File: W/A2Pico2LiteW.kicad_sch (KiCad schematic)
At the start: 15 parts, among them J1 SolderJumper_2_Bridged, U1 RPI-Pico2

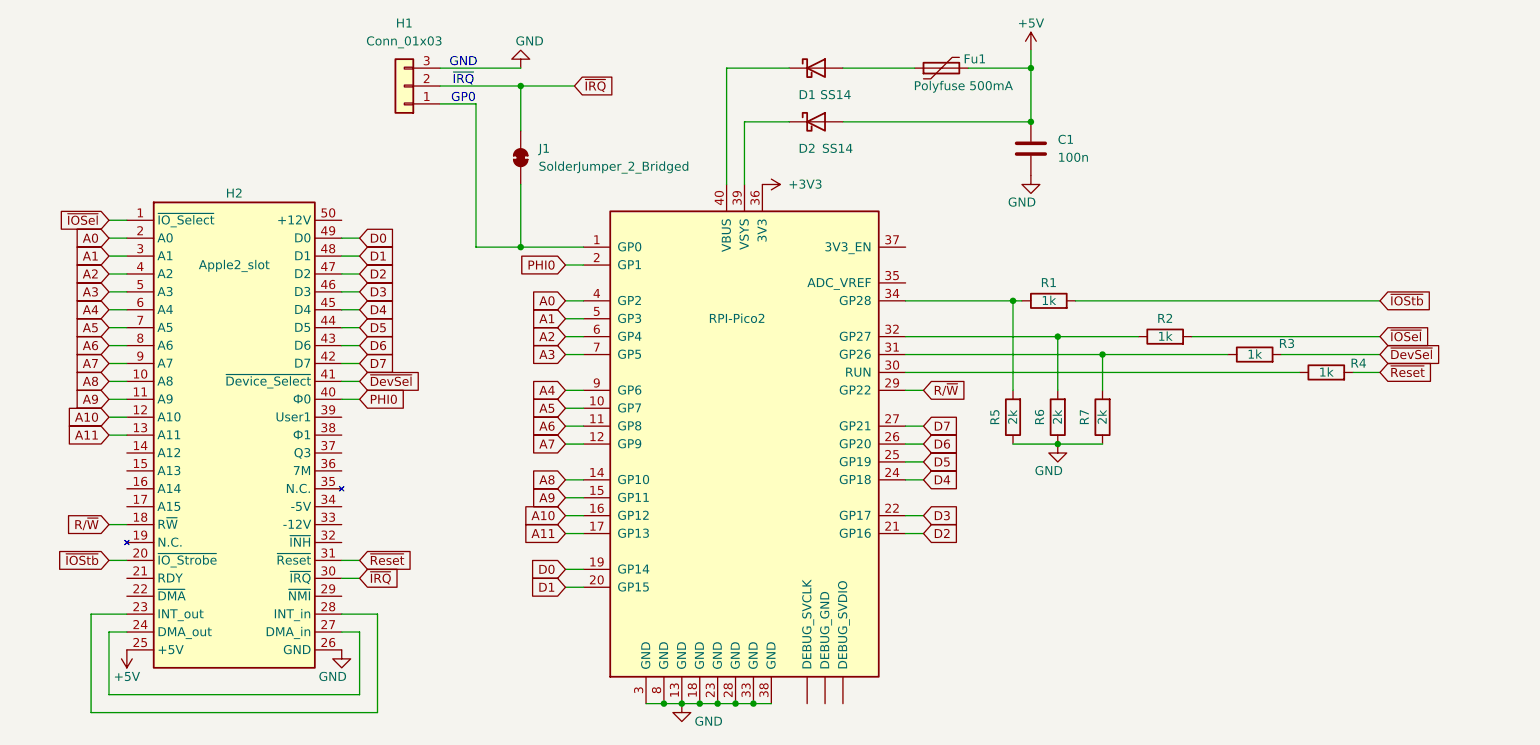
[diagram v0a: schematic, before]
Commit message: Add files via upload
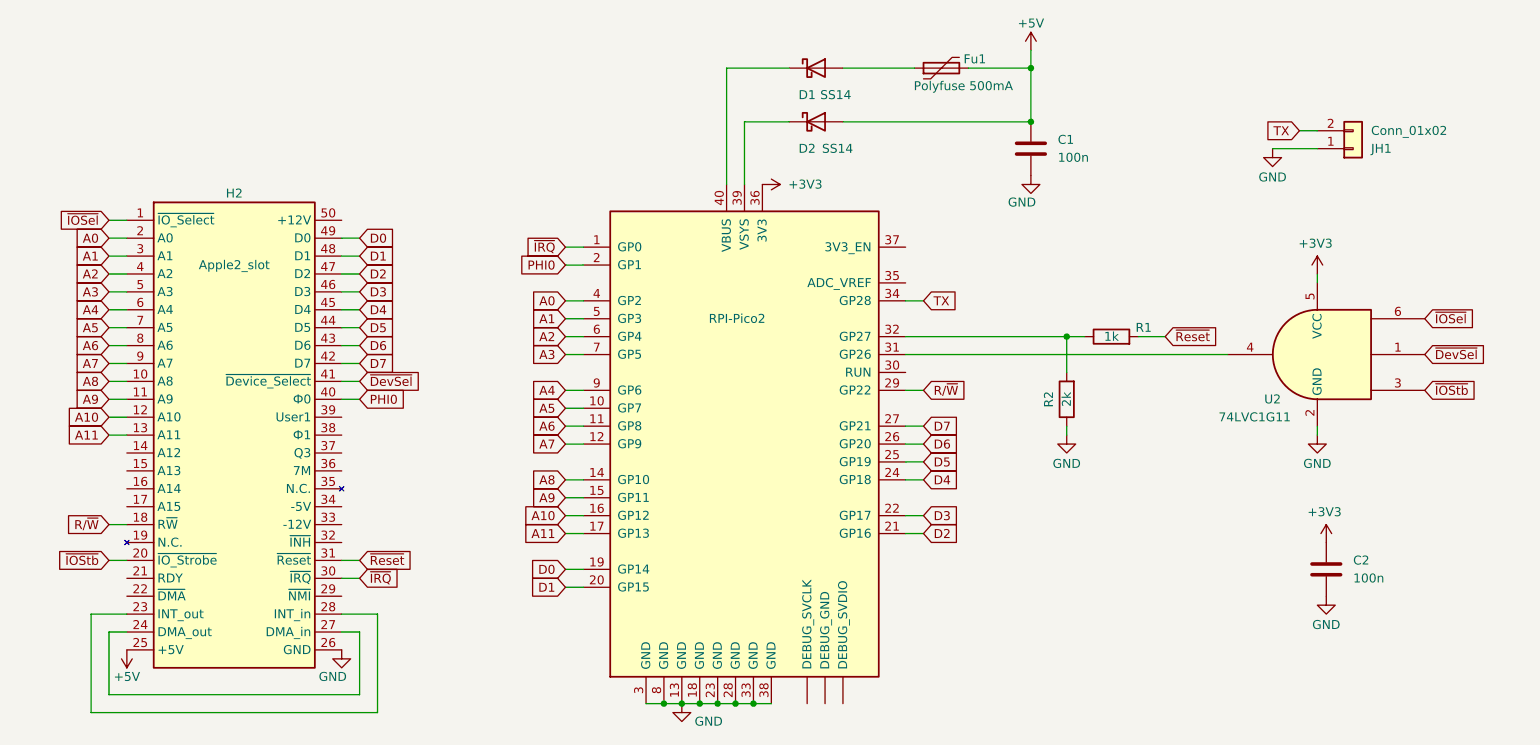
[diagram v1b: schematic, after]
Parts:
- removed H1: Conn_01x03, symbol Connector_Generic:Conn_01x03
- removed J1: SolderJumper_2_Bridged, symbol Jumper:SolderJumper_2_Bridged
- removed R1, R2, R3: 1k, Resistor_SMD:R_0402_1005Metric_Pad0.72x0.64mm_HandSolder, symbol Device:R
- removed R6, R7: 2k, Resistor_SMD:R_0402_1005Metric_Pad0.72x0.64mm_HandSolder, symbol Device:R
- added C2: 100n, symbol Device:C
- added JH1: Conn_01x02, symbol Connector_Generic:Conn_01x02
- added U2: 74LVC1G11, symbol 74xGxx:74LVC1G11
- renumbered R4 to R1, R5 to R2
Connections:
- net +3V3: now also C2.1, U2.5 (VCC)
- net GND: now also C2.2, JH1.1 (Pin_1), U2.2 (GND)
- net ~{DevSel}: now also U2.1
- net ~{IOSel}: now also U2.6
- net ~{IOStb}: now also U2.3
- net ~{IRQ}: now also U1.1 (GP0)
- net at U1.32 (GP27): now also R1.1, R2.2
- net at U1.31 (GP26): now also U2.4
- net TX: now reaches U1.34 (GP28)
- net TX: now also JH1.2 (Pin_2); no longer R2.2
- net at U1.30 (RUN): no longer R1.1
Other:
- note removed: "GND"
- note removed: "GP0"
- note removed: "~{IRQ}"
- moved on the sheet: R1, R2
